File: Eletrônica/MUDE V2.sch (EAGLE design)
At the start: 36 parts, among them J1 22-05-7038-03, J2 22-05-7038-03, Q1 MOSFET-NCHANNEL2N7002PW, Q2 MOSFET-NCHANNEL2N7002PW, Q3 MOSFET-NCHANNEL2N7002PW, Q4 MOSFET-NCHANNEL2N7002PW, Q5 MOSFET-NCHANNEL2N7002PW, U2 Tiny85-20-SMT

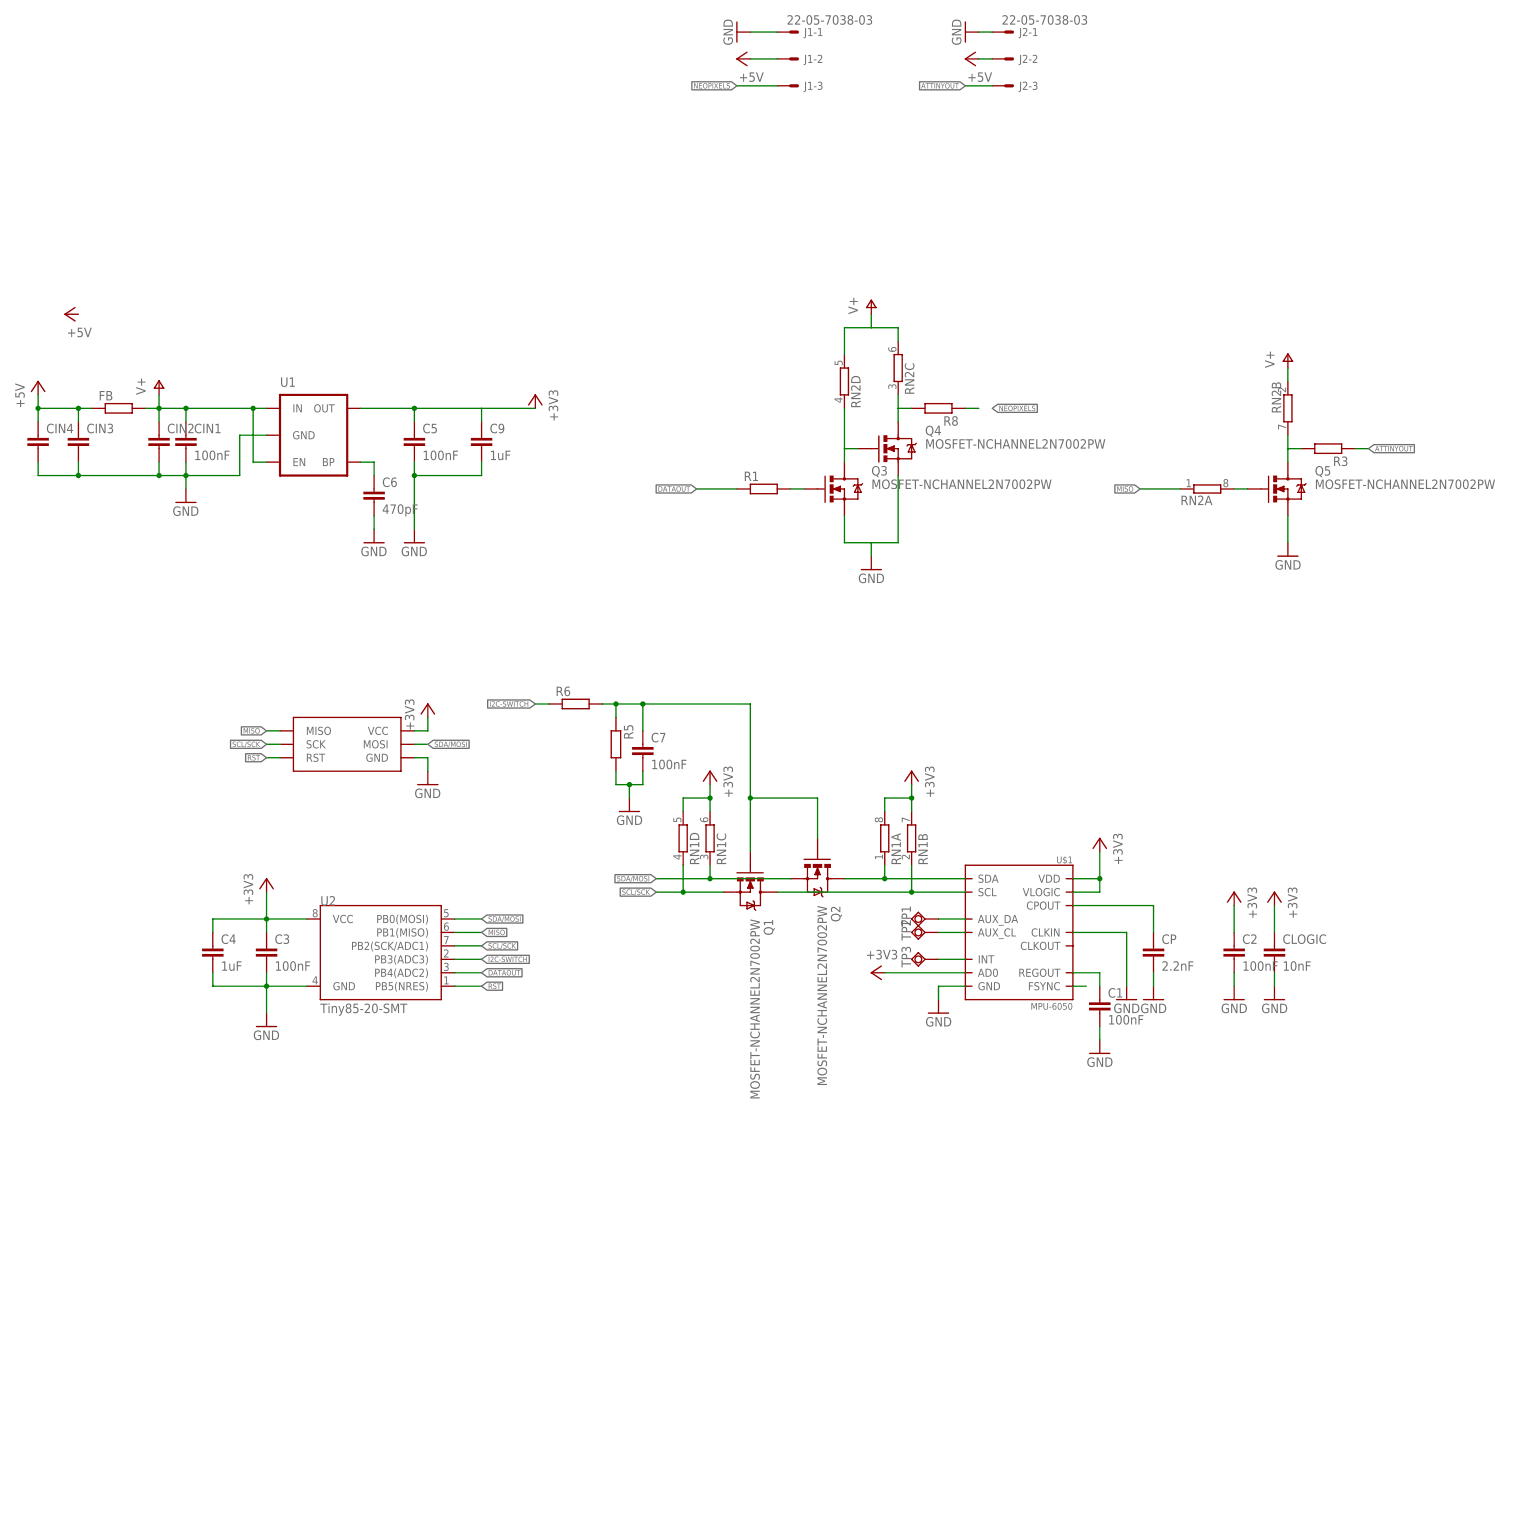
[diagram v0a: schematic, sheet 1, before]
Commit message: MUDE V2 files
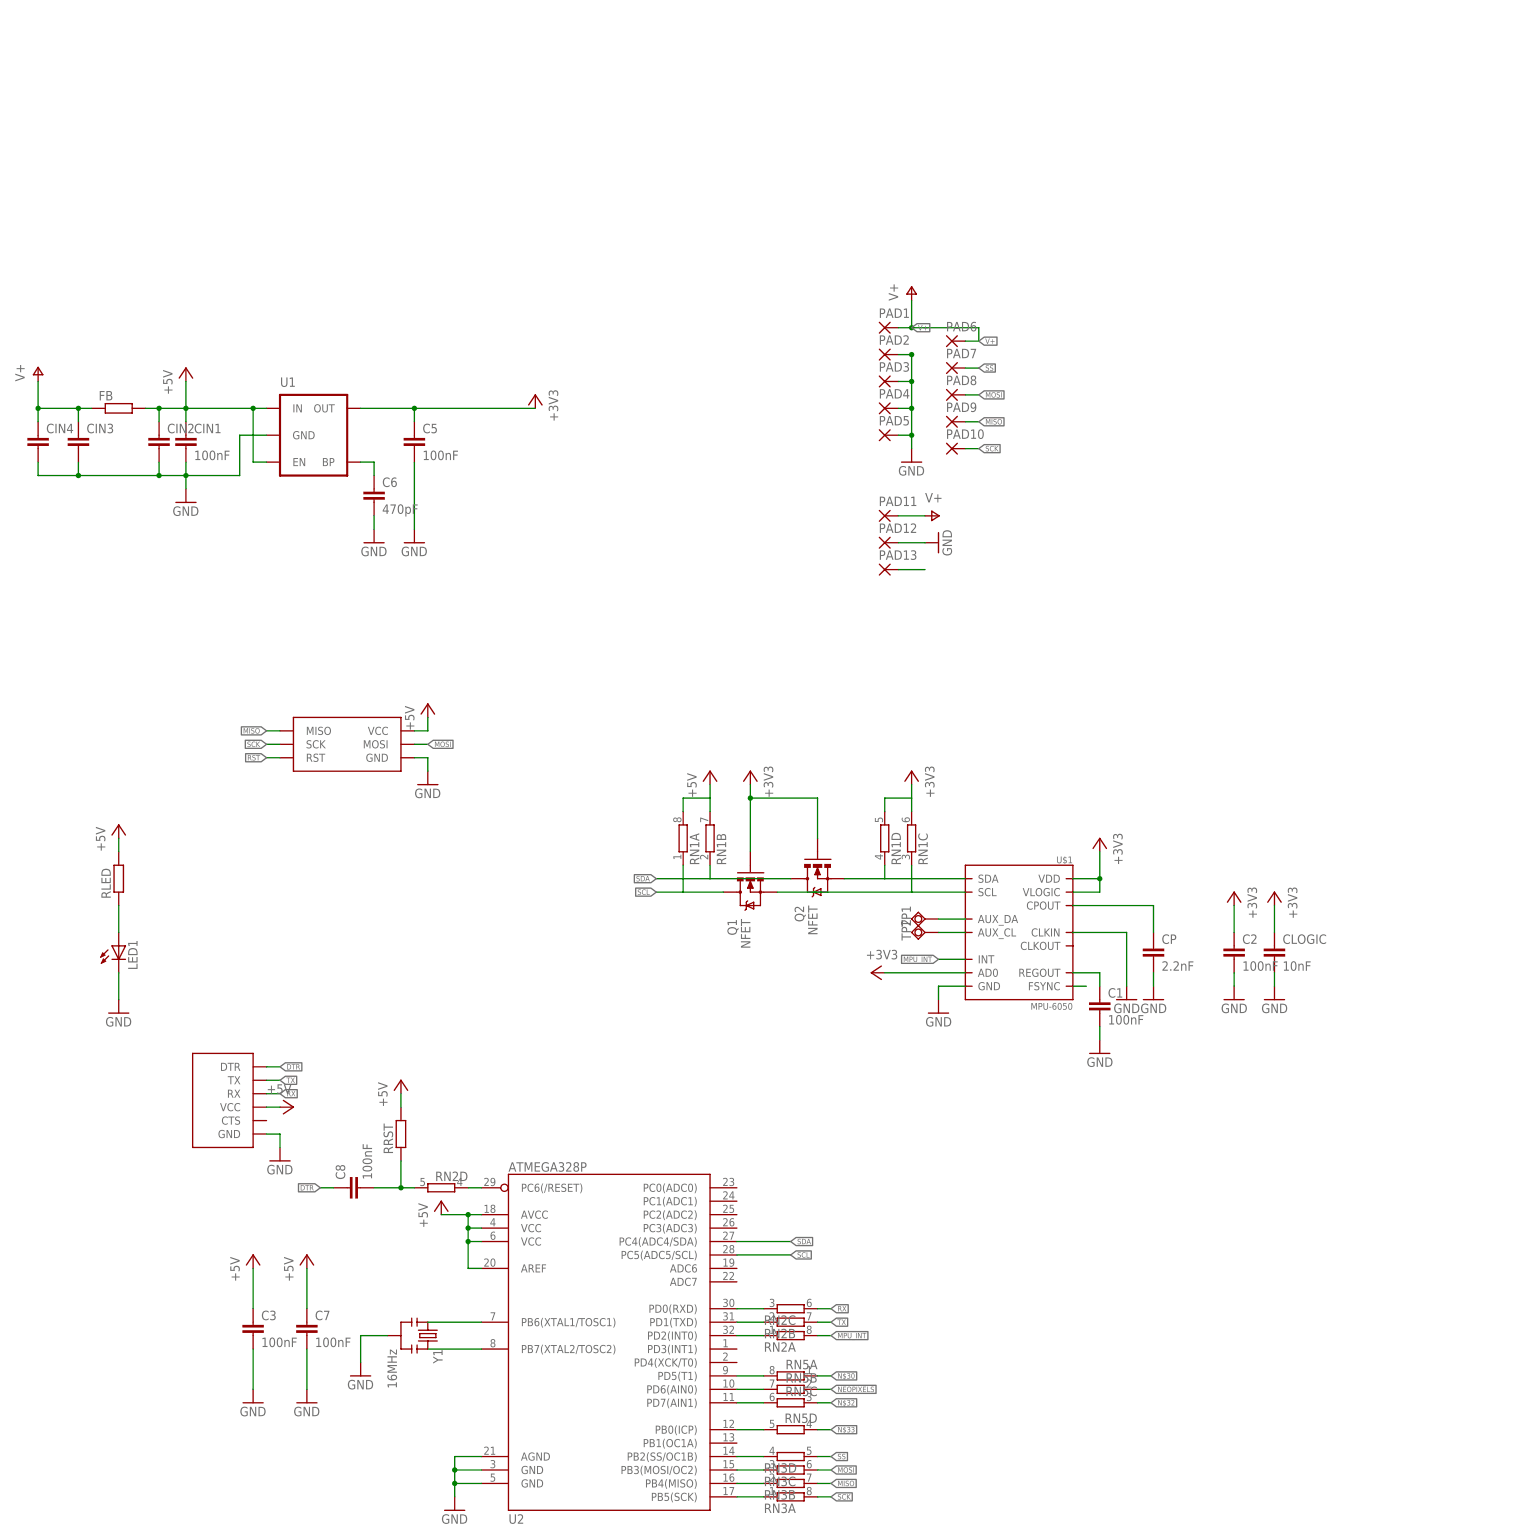
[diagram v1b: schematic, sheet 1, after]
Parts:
- removed C4, C9: 1uF, wes:C-EUC0603
- removed J1, J2: 22-05-7038-03, con-molex:22-05-7038-03
- removed Q3, Q4, Q5: MOSFET-NCHANNEL2N7002PW, SparkFun-DiscreteSemi:MOSFET-NCHANNEL2N7002PW
- removed R1, R3, R5, R6, R8: (no value), wes:R-EU_R0603
- removed TP3: TPSQTP10R, testpad:TPSQTP10R
- added C8: 100nF, wes:C-EUC0603
- added LED1: (no value), SparkFun-LED:LED0603
- added PAD1, PAD10, PAD11, PAD12, PAD13, PAD2, PAD3, PAD4, PAD5, PAD6, PAD7, PAD8, PAD9: (no value), wirepad:SMD2
- added RLED, RRST: (no value), wes:R-EU_R0603
- added RN3, RN5: (no value), resistor-dil:4R-N0603-ARV
- added U$2: FTDI_HEADERSMD, wes:FTDI_HEADERSMD
- added Y1: 16MHz, SparkFun-FreqCtrl:RESONATOR16MHZ
- CIN3, CIN4: device wes:C-EUC0805 -> wes:C-EUC1210
- Q1, Q2: value MOSFET-NCHANNEL2N7002PW -> NFET; device SparkFun-DiscreteSemi:MOSFET-NCHANNEL2N7002PW -> SparkFun-DiscreteSemi:MOSFET-NCHANNELBSS123LT1G
- U$3: value ISP_POGOISP_LHOLE -> ISP_POGOISP_POGO; device wes:ISP_POGOISP_LHOLE -> wes:ISP_POGOISP_POGO
- U2: value Tiny85-20-SMT -> ATMEGA328P; device SparkFun-DigitalIC:ATTINY45TINY85-20-SMT -> SparkFun-DigitalIC:ATMEGA328_SMT
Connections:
- removed net ATTINYOUT: J2-3.S, R3.1
- removed net DATAOUT: R1.1, U2.PB4(ADC2)
- removed net I2C-SWITCH: R6.1, U2.PB3(ADC3)
- removed net N$17: C7.1, Q1.G, Q2.G, R5.1, R6.2
- removed net N$21: Q4.D, R8.2, RN2C.1
- removed net SCL/SCK: Q1.S, RN1D.1, U$3.SCK, U2.PB2(SCK/ADC1)
- removed net SDA/MOSI: Q2.S, RN1C.1, U$3.MOSI, U2.PB0(MOSI)
- removed net VIN: CIN3.1, CIN4.1, FB.1, J1-2.S, J2-2.S
- new net +5V: C3.1, C7.1, CIN1.1, CIN2.1, FB.2, RLED.2, RN1A.2, RN1B.2, RRST.2, U$2.VCC, U$3.VCC, U1.EN, U1.IN, U2.AREF, U2.AVCC, U2.VCC@1, U2.VCC@2
- new net DTR: C8.1, U$2.DTR
- new net MOSI: PAD8.P, RN3C.2, U$3.MOSI
- new net MPU_INT: RN2A.2, U$1.INT
- new net N$10: U2.PB6(XTAL1/TOSC1), Y1.1
- new net N$15: U2.PB7(XTAL2/TOSC2), Y1.3
- new net N$19: RN2D.1, U2.PC6(/RESET)
- new net N$20: RN5C.2, U2.PD7(AIN1)
- new net N$22: RN3A.1, U2.PB5(SCK)
- new net N$23: RN3B.1, U2.PB4(MISO)
- new net N$24: RN3C.1, U2.PB3(MOSI/OC2)
- new net N$25: RN3D.1, U2.PB2(SS/OC1B)
- new net N$26: RN5D.2, U2.PB0(ICP)
- new net N$29: C8.2, RN2D.2, RRST.1
- new net N$30: RN5A.1
- new net N$32: RN5C.1
- new net N$33: RN5D.1
- new net N$8: RN5A.2, U2.PD5(T1)
- new net RX: RN2C.2, U$2.RX
- new net SCK: PAD10.P, RN3A.2, U$3.SCK
- new net SCL: Q1.D, RN1A.1, U2.PC5(ADC5/SCL)
- new net SDA: Q2.D, RN1B.1, U2.PC4(ADC4/SDA)
- new net SS: PAD7.P, RN3D.2
- new net TX: RN2B.2, U$2.TX
- net +3V3: now also Q1.G, Q2.G; no longer C3.1, C4.1, C9.1, RN1A.2, RN1B.2, U$3.VCC, U2.VCC
- net GND: now also LED1.C, PAD12.P, PAD2.P, PAD3.P, PAD4.P, PAD5.P, U$2.GND, U2.AGND, U2.GND@1, U2.GND@2, Y1.2; no longer C4.2, C9.2, J1-1.S, J2-1.S, Q3.S, Q4.S, Q5.S, R5.2, U2.GND
- net MISO: now also PAD9.P, RN3B.2; no longer RN2A.1, U2.PB1(MISO)
- net N$11: now also LED1.A, RLED.1; no longer TP3.TP, U$1.INT
- net N$14: now also RN2B.1, U2.PD1(TXD); no longer Q3.G, R1.2
- net N$16: now also RN5B.2, U2.PD6(AIN0); no longer Q3.D, Q4.G, RN2D.1
- net N$18: now also RN2A.1, U2.PD2(INT0); no longer Q5.D, R3.2, RN2B.2
- net N$2: now also RN2C.1, U2.PD0(RXD); no longer Q5.G, RN2A.2
- net N$7: now also Q2.S, RN1D.1; no longer Q2.D, RN1A.1
- net N$9: now also Q1.S, RN1C.1; no longer Q1.D, RN1B.1
- net NEOPIXELS: now also PAD13.P, RN5B.1; no longer J1-3.S, R8.1
- net RST: no longer U2.PB5(NRES)
- net V+: now also CIN3.1, CIN4.1, FB.1, PAD1.P, PAD11.P, PAD6.P; no longer CIN1.1, CIN2.1, FB.2, RN2B.1, RN2C.2, RN2D.2, U1.EN, U1.IN
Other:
- moved on the sheet: C3, C7, RN1A, RN1B, RN1C, RN1D, RN2A, RN2B, RN2C, RN2D
